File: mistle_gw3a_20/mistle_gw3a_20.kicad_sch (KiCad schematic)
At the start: 53 parts, among them J1 SWD, J2 USB_C_Receptacle_USB2.0, SW1 Boot, U1 SY8113BADC, U2 W25Q64JVS, U3 USBLC6-2SC6, U4 RP2040, Y1 12MHz

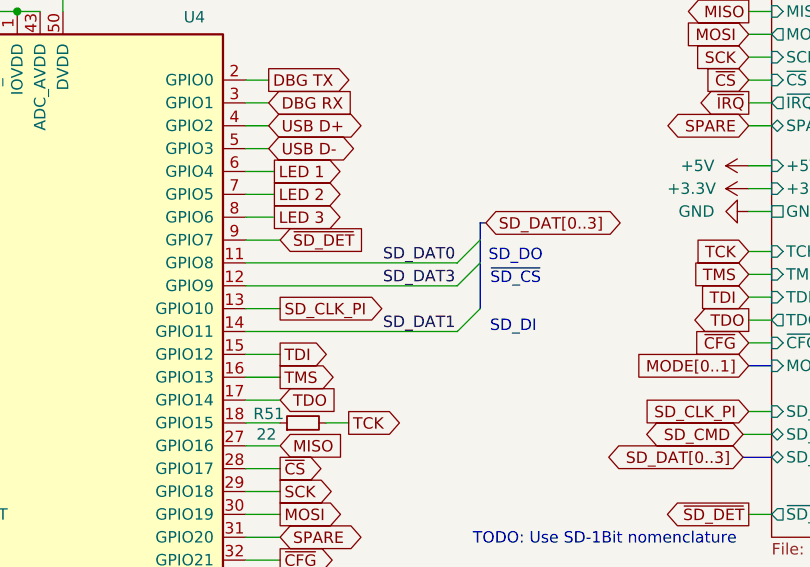
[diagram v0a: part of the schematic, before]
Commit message: Update gw3a dev board
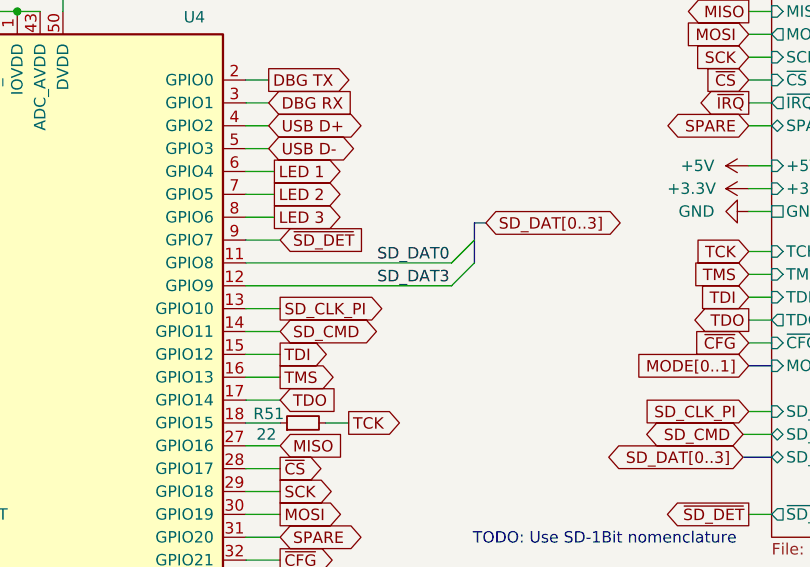
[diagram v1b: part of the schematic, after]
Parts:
- C1, C10, C11, C12, C13, C14, C2, C3, C5, C51, C52, C53, C54, C55, C56, C57, C6, C7, C8, C9, D1, D2, D3, D4, J1, J2, L3, R1, R10, R11, R12, R2, R3, R4, R5, R51, R54, R55, R6, R7, R8, R9, SW1, U1, U3, U4, Y1: checked once -> (none)
- R53: LCSC Part # C11702 -> C25792; checked once -> (none)
- U2: footprint Package_SO:SOIC-8_5.23x5.23mm_P1.27mm -> Package_SO:SOIC-8_5.3x5.3mm_P1.27mm; LCSC Part # (none) -> C179171; checked once -> (none)
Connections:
- net SD_DAT1 is gone; now on net SD_CMD: U4.14 (GPIO11)
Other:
- note removed: "SD_DI"
- note removed: "SD_DO"
- note removed: "~{SD_CS}"
